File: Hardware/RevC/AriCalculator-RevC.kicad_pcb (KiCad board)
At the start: 2 copper layers, 76.2 x 147.3 mm, 126 parts, among them CON1 BDM, CON2 SPI, CON3 USB-MINI-B, IC1 MC9S12G, IC2 MCP1640, IC3 FT232RL, IC4 MCP1643, SW1 POWER SWITCH

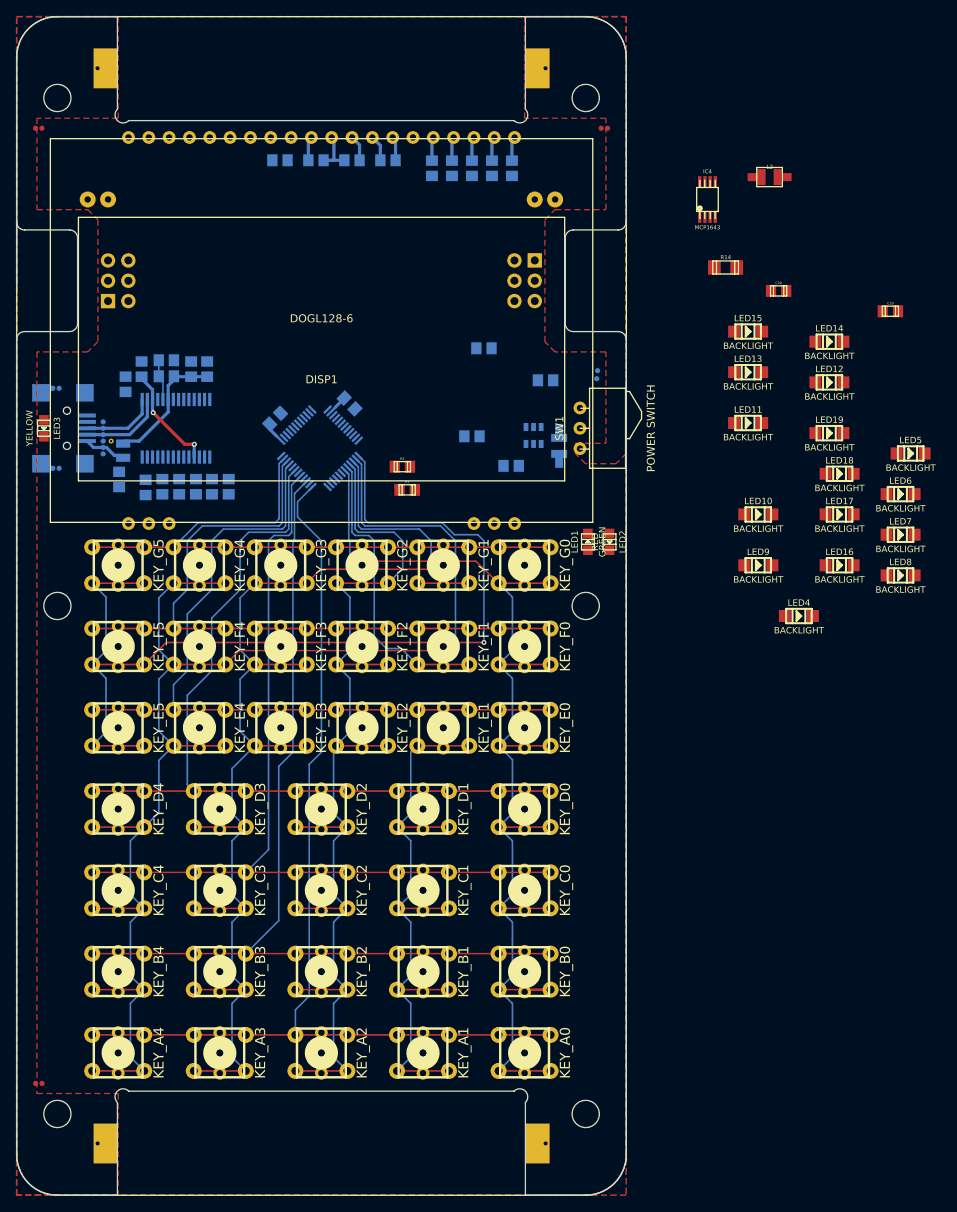
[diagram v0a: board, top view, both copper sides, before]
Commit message: work in progress
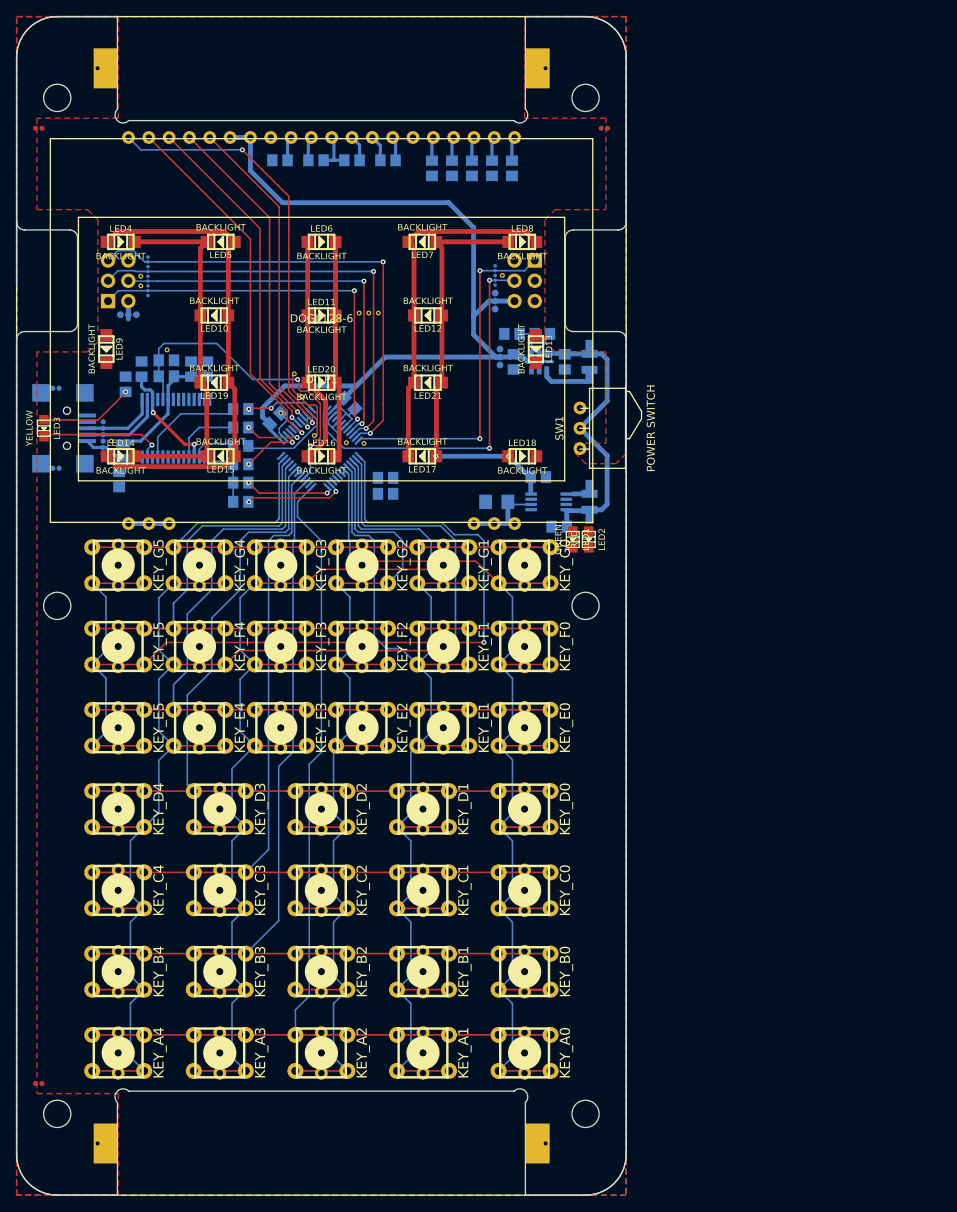
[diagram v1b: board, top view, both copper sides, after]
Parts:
- removed the spark_gap_pad_0.8 at (141.1, 111.3)
- removed the spark_gap_pad_0.8 at (141.2, 110.3)
- added ?: , VIA, B.Cu at (112.0, 119.4)
- added ?: , VIA, F.Cu at (104.2, 113.5)
- added ?: , VIA, F.Cu at (103.3, 110.7)
- added ?: , VIA, F.Cu at (105.8, 118.4)
- added ?: , VIA, F.Cu at (87.4, 107.7)
- added ?: , VIA, F.Cu at (111.4, 103.1)
- added ?: , VIA, F.Cu at (101.6, 115.6)
- added ?: , VIA, F.Cu at (112.6, 103.1)
- added ?: , VIA, F.Cu at (129.3, 98.4)
- added ?: , VIA, F.Cu at (84.1, 99.7)
- added ?: , VIA, F.Cu at (84.1, 98.5)
- added ?: , VIA, F.Cu at (113.8, 103.1)
- added ?: , VIA, B.Cu at (109.8, 119.3)
- added spark_gap_pad_0.6: SG, spark_gap_pad_0.6, B.Cu at (85.0, 98.5)
- added spark_gap_pad_0.6: SG, spark_gap_pad_0.6, B.Cu at (128.4, 98.4)
- added spark_gap_pad_0.6: SG, spark_gap_pad_0.6, B.Cu at (128.4, 97.8)
- added spark_gap_pad_0.6: SG, spark_gap_pad_0.6, B.Cu at (128.4, 97.2)
- added spark_gap_pad_0.6: SG, spark_gap_pad_0.6, B.Cu at (128.4, 99.0)
- added spark_gap_pad_0.6: SG, spark_gap_pad_0.6, B.Cu at (128.4, 99.6)
- added spark_gap_pad_0.6: SG, spark_gap_pad_0.6, B.Cu at (85.0, 97.9)
- added spark_gap_pad_0.6: SG, spark_gap_pad_0.6, B.Cu at (85.0, 99.1)
- added spark_gap_pad_0.6: SG, spark_gap_pad_0.6, B.Cu at (85.0, 99.7)
- added spark_gap_pad_0.6: SG, spark_gap_pad_0.6, B.Cu at (85.0, 100.3)
- added spark_gap_pad_0.6: SG, spark_gap_pad_0.6, B.Cu at (85.0, 100.9)
- added spark_gap_pad_0.6: SG, spark_gap_pad_0.6, B.Cu at (85.0, 97.3)
- added spark_gap_pad_0.6: SG, spark_gap_pad_0.6, B.Cu at (85.0, 96.7)
- added spark_gap_pad_0.6: SG, spark_gap_pad_0.6, B.Cu at (85.0, 96.1)
- added spark_gap_pad_1.0: SG, spark_gap_pad_1.0, B.Cu at (129.0, 108.6)
- added spark_gap_pad_1.0: SG, spark_gap_pad_1.0, B.Cu at (129.0, 107.6)
- added spark_gap_pad_1.0: SG, spark_gap_pad_1.0, B.Cu at (129.0, 109.6)
- added spark_gap_pad_1.0: SG, spark_gap_pad_1.0, B.Cu at (82.5, 103.3)
- added spark_gap_pad_1.0: SG, spark_gap_pad_1.0, B.Cu at (83.5, 103.3)
- added spark_gap_pad_1.0: SG, spark_gap_pad_1.0, B.Cu at (81.5, 103.3)
- added spark_gap_pad_1.0: SG, spark_gap_pad_1.0, B.Cu at (128.4, 101.6)
- added spark_gap_pad_1.0: SG, spark_gap_pad_1.0, B.Cu at (128.4, 100.6)
- added spark_gap_pad_1.0: SG, spark_gap_pad_1.0, B.Cu at (128.4, 102.6)
- C19, C20, IC4, L2, R1, R14, R2: moved to B.Cu
- LED20, LED21: value IR -> BACKLIGHT; footprint led_5mm_bend -> Led_1206; moved to F.Cu
- moved LED4 96.8 mm to (81.6, 94.2)
- moved LED5 90.2 mm to (94.1, 94.2), turned to 180 degrees
- moved LED14 89.7 mm to (81.6, 121.0)
- moved LED9 85.9 mm to (79.8, 107.6), turned to 270 degrees
- moved LED6 78.9 mm to (106.7, 94.2)
- moved LED19 77.1 mm to (93.3, 111.8), turned to 180 degrees
- moved LED10 72.4 mm to (93.3, 103.4), turned to 180 degrees
- moved LED7 70.1 mm to (119.3, 94.2), turned to 180 degrees
- moved LED15 67.7 mm to (94.1, 121.0), turned to 180 degrees
- moved LED16 66.2 mm to (106.7, 121.0)
- moved LED8 63.0 mm to (131.8, 94.2)
- moved LED11 55.0 mm to (106.7, 103.4)
- moved LED17 52.7 mm to (119.3, 121.0), turned to 180 degrees
- moved LED12 50.9 mm to (120.0, 103.4), turned to 180 degrees
- moved C19 49.4 mm to (136.4, 129.8)
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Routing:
- net N-0000068: track 0.00 -> 147.0 mm, vias 0 -> 2
- net N-0000067: track 0.00 -> 127.7 mm
- net 3V3: track 5.17 -> 114.5 mm
- net N-0000034: track 0.00 -> 59.6 mm, vias 0 -> 2
- net N-0000031: track 0.00 -> 55.8 mm, vias 0 -> 2
- net /Display/DISPLAY_SS: track 0.00 -> 53.8 mm, vias 0 -> 2
- net N-0000030: track 0.00 -> 49.4 mm, vias 0 -> 2
- net N-0000026: track 0.00 -> 49.3 mm, vias 0 -> 2
- net N-0000045: track 0.00 -> 48.4 mm, vias 0 -> 2
- net /Display/DISPLAY_RESET: track 0.00 -> 46.1 mm, vias 0 -> 1
- net N-0000033: track 0.00 -> 43.6 mm, vias 0 -> 2
- net /Display/DISPLAY_A0: track 0.00 -> 42.5 mm, vias 0 -> 1
- net /Display/DISPLAY_MOSI: track 0.00 -> 42.4 mm, vias 0 -> 1
- net /Display/DISPLAY_SCK: track 0.00 -> 41.0 mm, vias 0 -> 1
- net +BATT: track 0.00 -> 36.4 mm
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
